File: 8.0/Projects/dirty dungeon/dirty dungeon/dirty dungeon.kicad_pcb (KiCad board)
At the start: 2 copper layers, 149.9 x 81.3 mm, 136 parts, among them J1 sensPin1, J10 sensPin1, J11 sensPin1, J12 sensPin1, J13 sensPin1, J14 sensPin1, J15 sensPin1, J16 sensPin1, J17 sensPin1, J18 sensPin1, J19 sensPin1, J2 sensPin2, J20 sensPin1, J21 sensPin1, J22 sensPin1, J25 5VDC, J3 sensPin3, J4 sensPin4, J5 sensPin1, J6 sensPin1, J7 sensPin1, J8 sensPin1, J9 sensPin1, Q1 IRLML6244, Q10 IRLML6244, Q11 IRLML6244, Q12 IRLML6244, Q13 IRLML6244, Q14 IRLML6244, Q15 IRLML6244, Q16 IRLML6244, Q17 IRLML6244, Q18 IRLML6244, Q19 IRLML6244, Q2 IRLML6244, Q20 IRLML6244, Q21 IRLML6244, Q22 IRLML6244, Q3 IRLML6244, Q4 IRLML6244, Q5 IRLML6244, Q6 IRLML6244, Q7 IRLML6244, Q8 IRLML6244, Q9 IRLML6244, U1 ESP32-WROOM-32D, U2 OKI-78SR-3.3_1.5-W36H-C

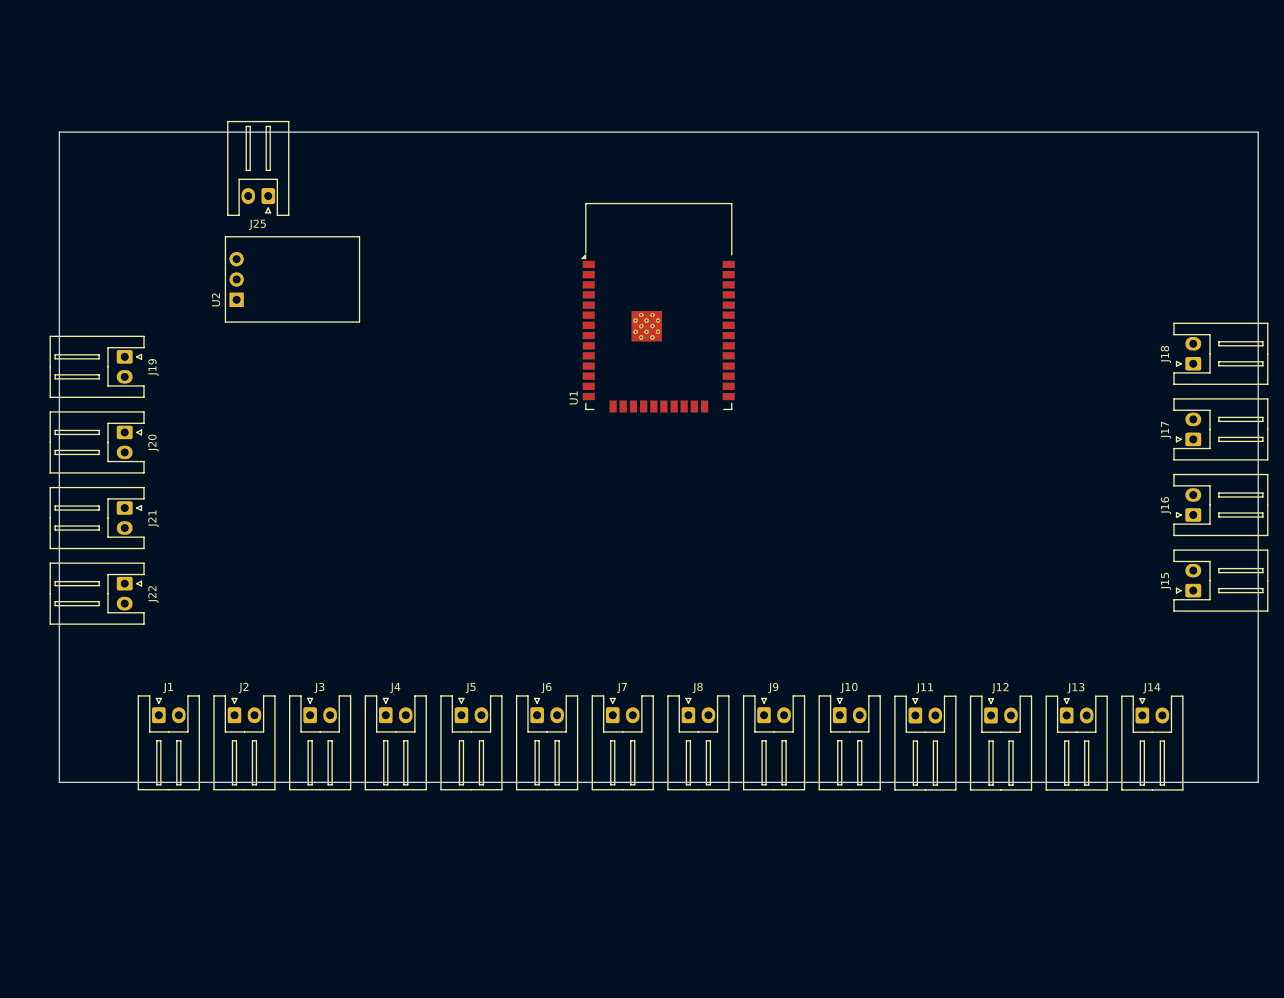
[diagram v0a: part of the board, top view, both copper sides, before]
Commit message: fh
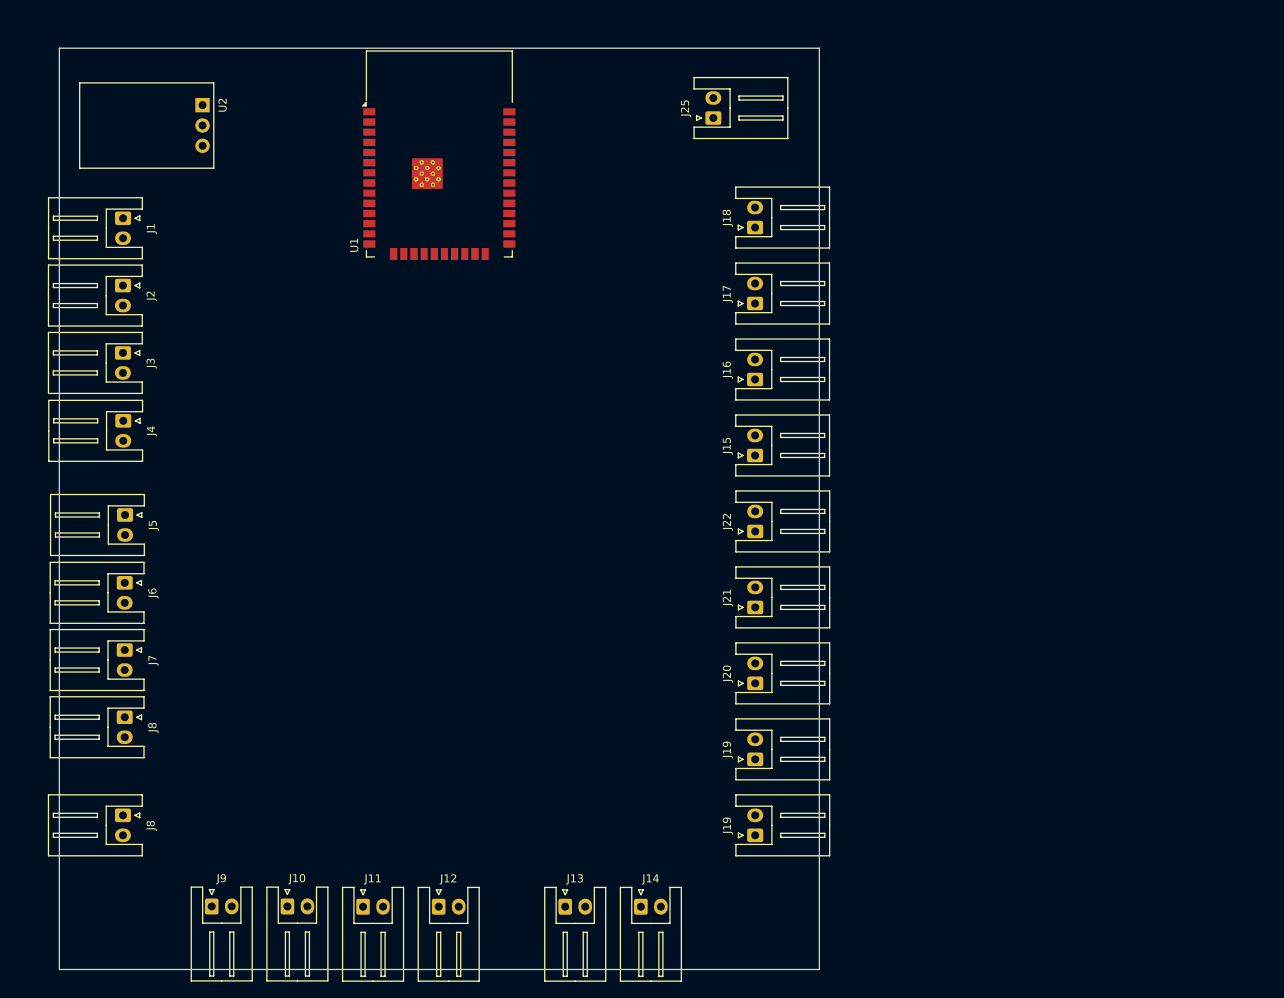
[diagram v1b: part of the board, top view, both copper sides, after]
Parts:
- added J19: sensPin1, Connector_JST:JST_XH_S2B-XH-A_1x02_P2.50mm_Horizontal, F.Cu at (158.1, 143.8)
- added J8: sensPin1, Connector_JST:JST_XH_S2B-XH-A_1x02_P2.50mm_Horizontal, F.Cu at (79.1, 141.3)
- moved J19 93.5 mm to (158.1, 134.3), turned to 90 degrees
- moved J20 84.8 mm to (158.1, 124.8), turned to 90 degrees
- moved J21 79.8 mm to (158.1, 115.3), turned to 90 degrees
- moved J22 79.1 mm to (158.1, 105.8), turned to 90 degrees
- moved J10 73.1 mm to (99.6, 152.7)
- moved J11 73.1 mm to (109.1, 152.7)
- moved J12 73.1 mm to (118.5, 152.7)
- moved J9 73.1 mm to (90.2, 152.7)
- moved J8 70.5 mm to (79.3, 129.0), turned to -90 degrees
- moved J13 67.1 mm to (134.4, 152.7)
- moved J14 67.1 mm to (143.8, 152.7)
- moved J1 62.3 mm to (79.1, 66.6), turned to -90 degrees
- moved J7 61.5 mm to (79.3, 120.6), turned to -90 degrees
- moved J18 57.4 mm to (158.1, 67.8)
- moved J17 57.4 mm to (158.1, 77.3)
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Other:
- board size 149.9 x 81.3 mm -> 95 x 115.2 mm
